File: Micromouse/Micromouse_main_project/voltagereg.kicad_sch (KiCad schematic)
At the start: 7 parts, among them U1 VL53L1CXV0FY1

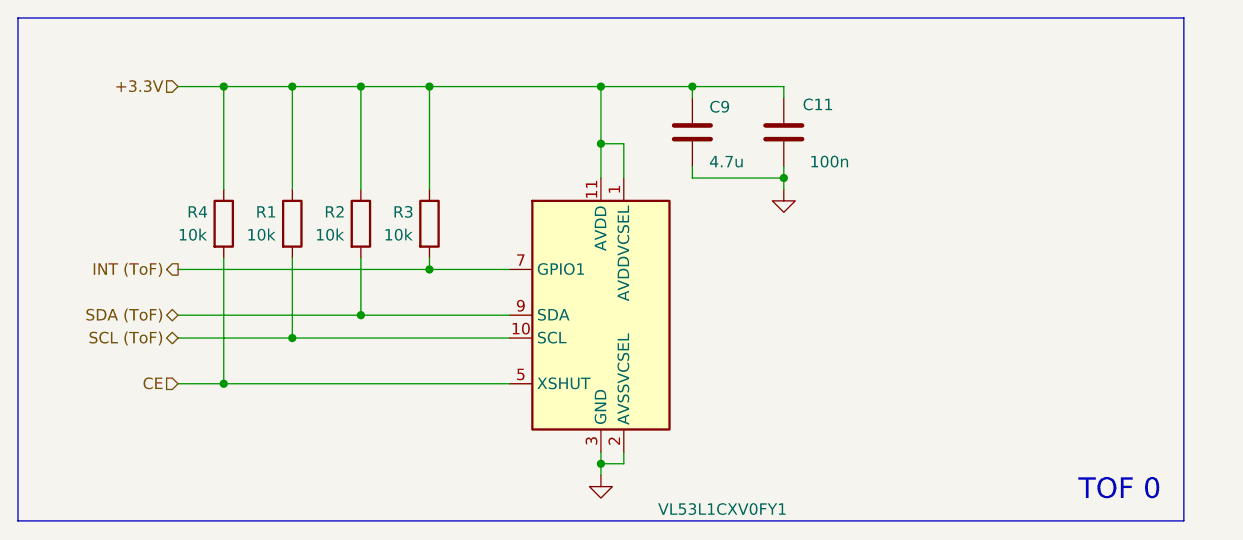
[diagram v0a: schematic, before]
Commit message: Schematic overhaul
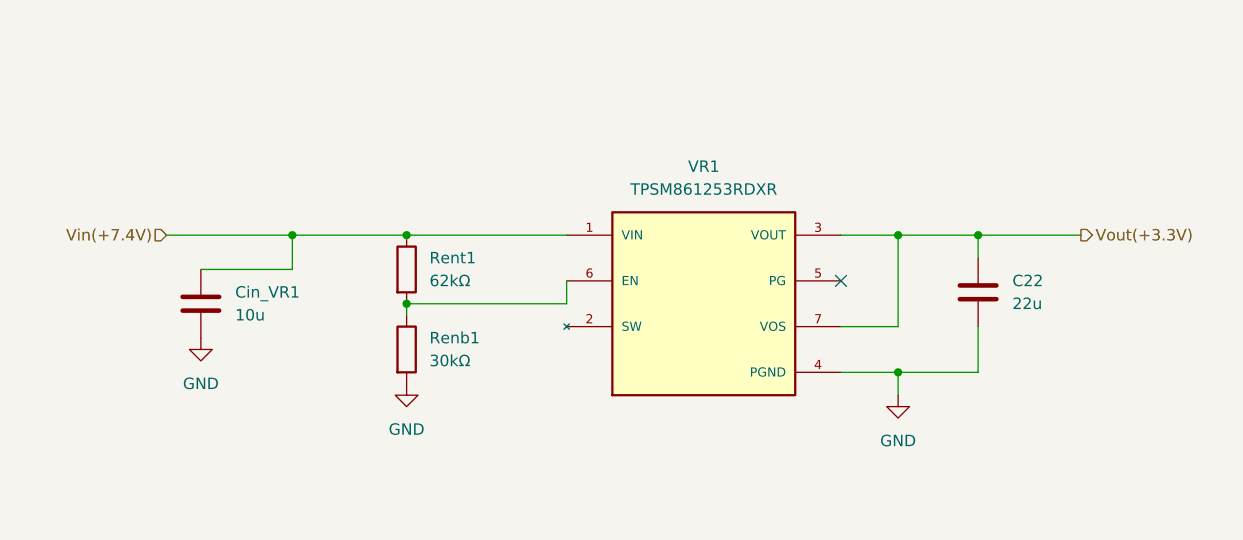
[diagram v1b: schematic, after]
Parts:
- removed C11: 100n, Capacitor_SMD:C_0402_1005Metric, symbol Device:C
- removed C9: 4.7u, Capacitor_SMD:C_0402_1005Metric, symbol Device:C
- removed R1, R2, R3, R4: 10k, Resistor_SMD:R_0603_1608Metric, symbol Device:R
- removed U1: VL53L1CXV0FY1, MM_VL53L4CDV0DH-1:LGA12_STM, symbol Sensor_Distance:VL53L1CXV0FY1
- added C22: 22u, Capacitor_SMD:C_0603_1608Metric, symbol Device:C
- added Cin_VR1: 10u, Capacitor_SMD:C_0603_1608Metric, symbol Device:C
- added Renb1: 30kΩ, Resistor_SMD:R_0603_1608Metric, symbol Device:R
- added Rent1: 62kΩ, Resistor_SMD:R_0603_1608Metric, symbol Device:R
- added VR1: TPSM861253RDXR, MM_TPSM861253RDXR:TPSM861253RDXR, symbol TPSM861253RDXR:TPSM861253RDXR
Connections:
- net GND: now also C22.2, Cin_VR1.2, Renb1.2, VR1.4 (PGND)
- new net: Renb1.1, Rent1.2, VR1.6 (EN)
- new net Vin(+7.4V): Cin_VR1.1, Rent1.1, VR1.1 (VIN)
- new net Vout(+3.3V): C22.1, VR1.3 (VOUT), VR1.7 (VOS)
- no-connect marks 0 -> 1
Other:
- note removed: "TOF 0"

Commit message: Prepped layout
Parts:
- VR1: footprint MM_TPSM861253RDXR:TPSM861253RDXR -> TPSM862253RDXR_FOOTPRINT:TPSM861253RDXR
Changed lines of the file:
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@@
 			)
 		)
-		(property "Footprint" "MM_TPSM861253RDXR:TPSM861253RDXR"
+		(property "Footprint" "TPSM862253RDXR_FOOTPRINT:TPSM861253RDXR"
 			(at 139.7 97.79 0)
 			(hide yes)
